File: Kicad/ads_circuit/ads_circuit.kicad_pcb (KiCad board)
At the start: 2 copper layers, 50 x 35 mm, 5 parts, among them J1 Con

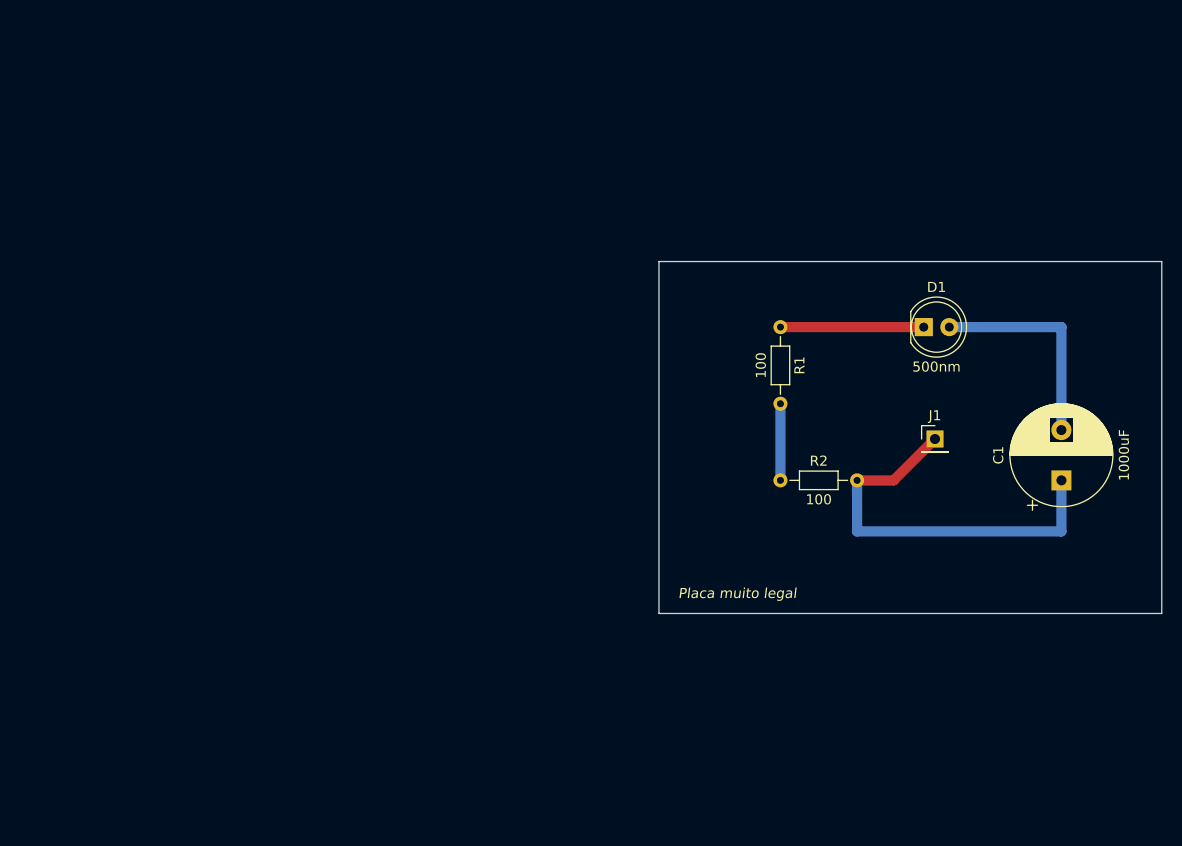
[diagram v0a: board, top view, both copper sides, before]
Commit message: Kicad scheme
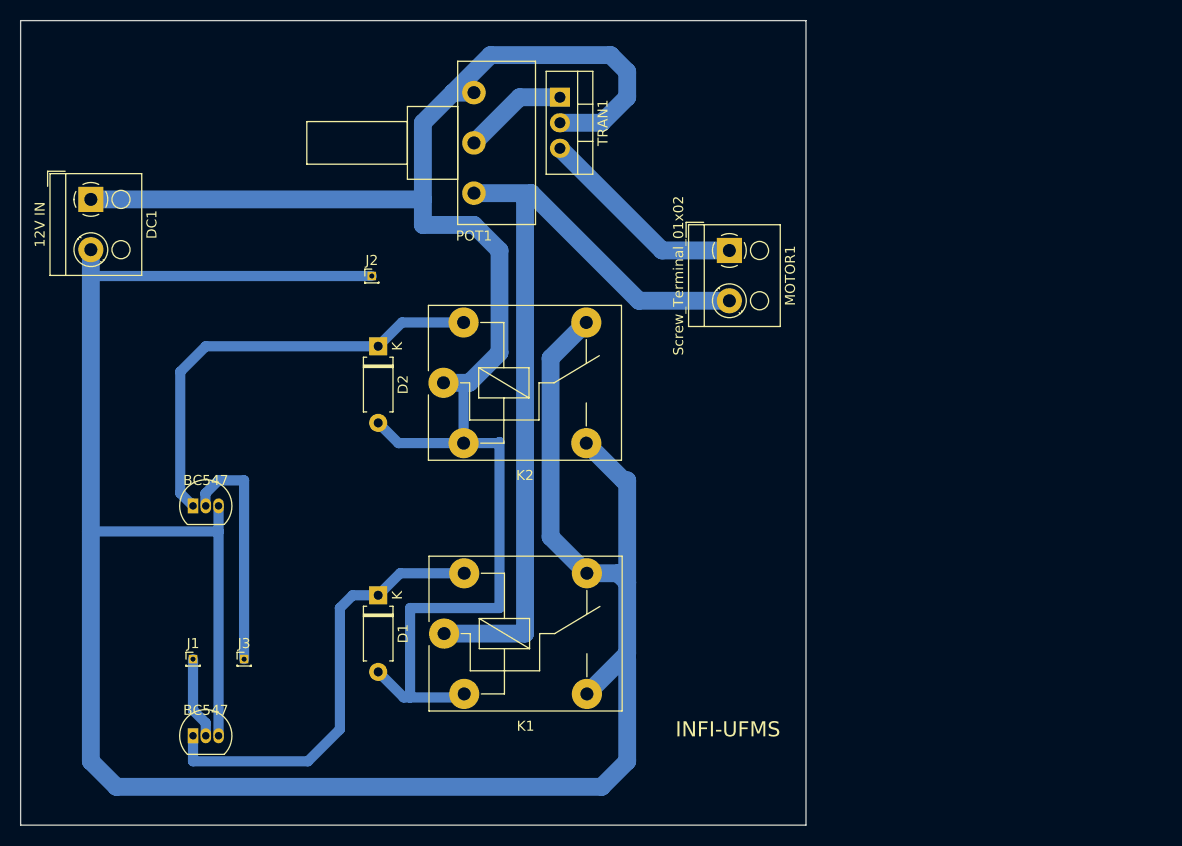
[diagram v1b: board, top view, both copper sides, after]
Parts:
- removed C1: 1000uF, Capacitor_THT:CP_Radial_D10.0mm_P5.00mm
- removed R1, R2: 100, Resistor_THT:R_Axial_DIN0204_L3.6mm_D1.6mm_P7.62mm_Horizontal
- added D2: DIODE, Diode_THT:D_A-405_P7.62mm_Horizontal, F.Cu at (92.1, 98.4)
- added DC1: 12V IN, TerminalBlock_RND:TerminalBlock_RND_205-00001_1x02_P5.00mm_Horizontal, F.Cu at (63.5, 83.8)
- added J2: ARDU GND, Connector_PinHeader_1.00mm:PinHeader_1x01_P1.00mm_Vertical, F.Cu at (91.4, 91.4)
- added J3: ARDU MOTOR 2, Connector_PinHeader_1.00mm:PinHeader_1x01_P1.00mm_Vertical, F.Cu at (78.7, 129.5)
- added K1: FINDER-36.11, Relay_THT:Relay_SPDT_Finder_36.11, F.Cu at (98.6, 127.0)
- added K2: FINDER-36.11, Relay_THT:Relay_SPDT_Finder_36.11, F.Cu at (98.6, 102.1)
- added MOTOR1: Screw_Terminal_01x02, TerminalBlock_RND:TerminalBlock_RND_205-00001_1x02_P5.00mm_Horizontal, F.Cu at (127.0, 88.9)
- added POT1: R_Potentiometer, Potentiometer_THT:Potentiometer_Piher_T-16H_Single_Horizontal, F.Cu at (101.6, 73.2)
- added Q1: BC547, Package_TO_SOT_THT:TO-92_Inline, F.Cu at (73.7, 137.2)
- added Q2: BC547, Package_TO_SOT_THT:TO-92_Inline, F.Cu at (73.7, 114.3)
- added TRAN1: TIP120, Package_TO_SOT_THT:TO-220-3_Vertical, F.Cu at (110.2, 73.7)
- D1: value 500nm -> DIODE; footprint LED_THT:LED_D5.0mm -> Diode_THT:D_A-405_P7.62mm_Horizontal
- J1: value Con -> ARDU MOTOR 1; footprint Connector_PinHeader_2.54mm:PinHeader_1x01_P2.54mm_Vertical -> Connector_PinHeader_1.00mm:PinHeader_1x01_P1.00mm_Vertical
- moved J1 77.0 mm to (73.7, 129.5)
- moved D1 60.5 mm to (92.1, 123.2), turned to -90 degrees
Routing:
- net Net-(DC1-Pad2): track 0.00 -> 240.8 mm
- net Net-(D1-Pad2): track 21.4 -> 168.2 mm
- net Net-(K1-Pad11): track 0.00 -> 81.9 mm
- net Net-(D2-Pad1): track 0.00 -> 44.1 mm
- net Net-(J1-Pad1): track 39.9 -> 8.15 mm
- net Net-(D1-Pad1): track 14.2 -> 44.3 mm
- net Net-(J3-Pad1): track 0.00 -> 23.4 mm
- net Net-(MOTOR1-Pad1): track 0.00 -> 21.1 mm
- net Net-(POT1-Pad2): track 0.00 -> 10.4 mm
- net Net-(R1-Pad2): track 7.62 -> 0.00 mm
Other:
- board size 50 x 35 mm -> 78.1 x 80 mm
- board text added: "INFI-UFMS"
- board text removed: "Placa muito legal"
